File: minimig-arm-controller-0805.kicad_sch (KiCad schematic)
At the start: 35 parts, among them CN1 USB_B_Mini, J1 Conn_02x03_Odd_Even, Q1 BC807, SW1 Reset, U1 AT91SAM7S256, U2 PIC_PIN_HEADER, X1 18.342MHz

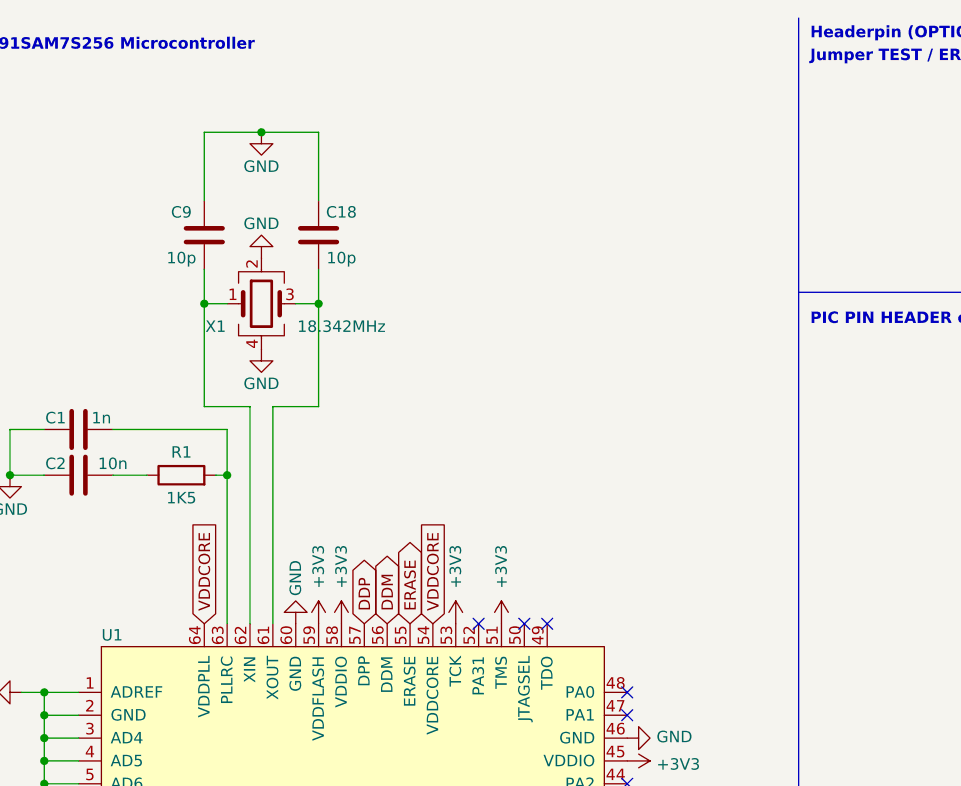
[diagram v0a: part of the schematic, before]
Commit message: latest rev. fix detached head and merge conflict.
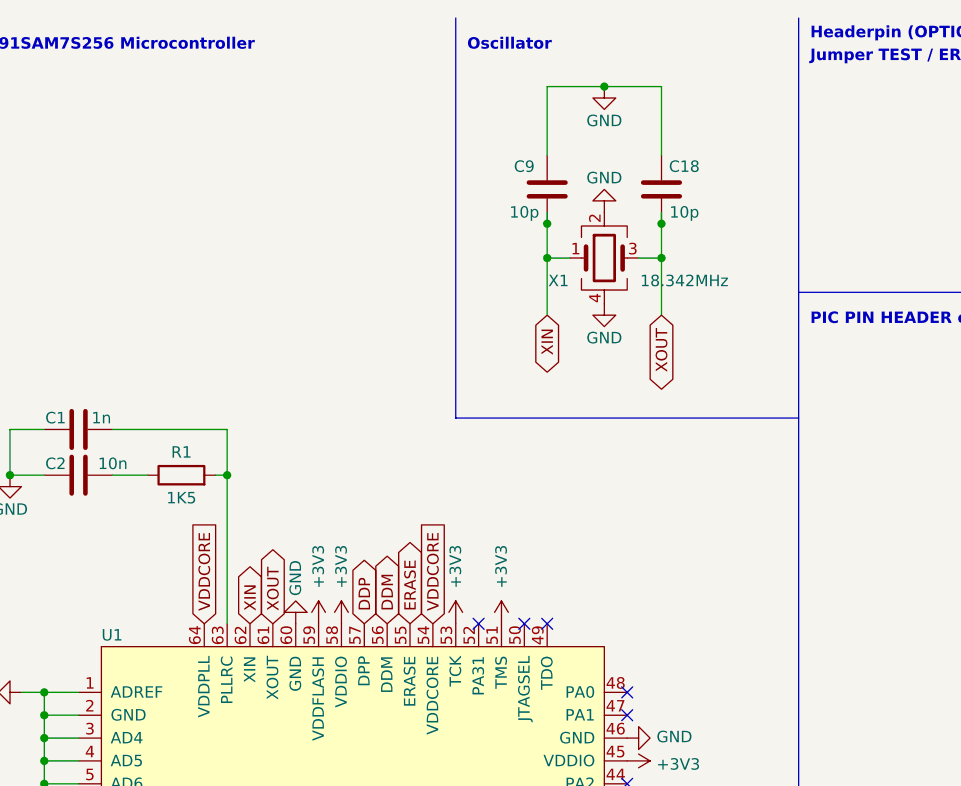
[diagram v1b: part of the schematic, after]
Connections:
- net XOUT: now reaches C18.1, U1.61 (XOUT), X1.3
- net XIN: now reaches C9.1, U1.62 (XIN), X1.1
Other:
- note added: "Oscillator"
- moved on the sheet: C18, C9, X1
